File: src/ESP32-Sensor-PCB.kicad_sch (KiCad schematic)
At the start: 3 parts, among them U1 XIAO-ESP32-S3-SMD, U2 HDC1080DMBR

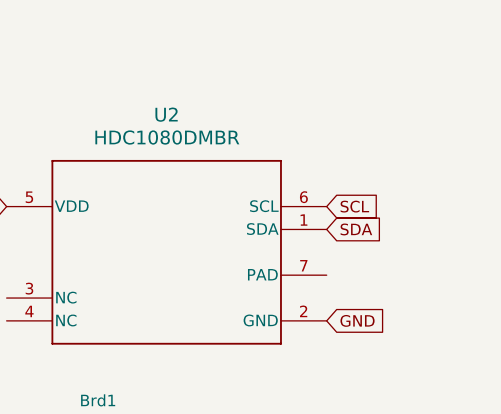
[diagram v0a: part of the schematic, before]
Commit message: lot
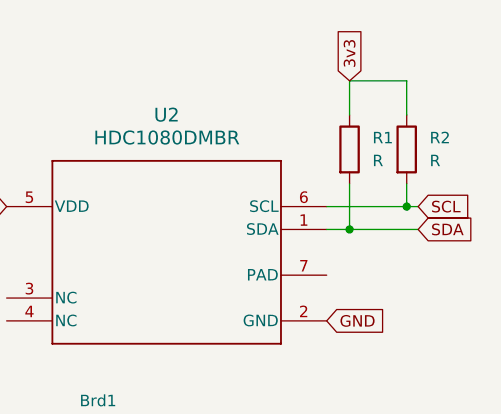
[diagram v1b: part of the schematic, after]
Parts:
- added R1, R2: R, symbol Device:R
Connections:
- net 3v3: now also R1.1, R2.1
- net SCL: now also R2.2
- net SDA: now also R1.2
